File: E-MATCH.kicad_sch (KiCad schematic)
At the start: 22 parts, among them IC1 NCV81071BZR2G, IC2 NCV81071BZR2G, J1 691210910002, J2 691210910002, J3 691210910002, J4 691210910002, J5 DC Jack, Q1 AOSP36326C, Q2 AOSP36326C, Q3 AOSP36326C, Q4 AOSP36326C, U1 TMCS1108A2UQDR

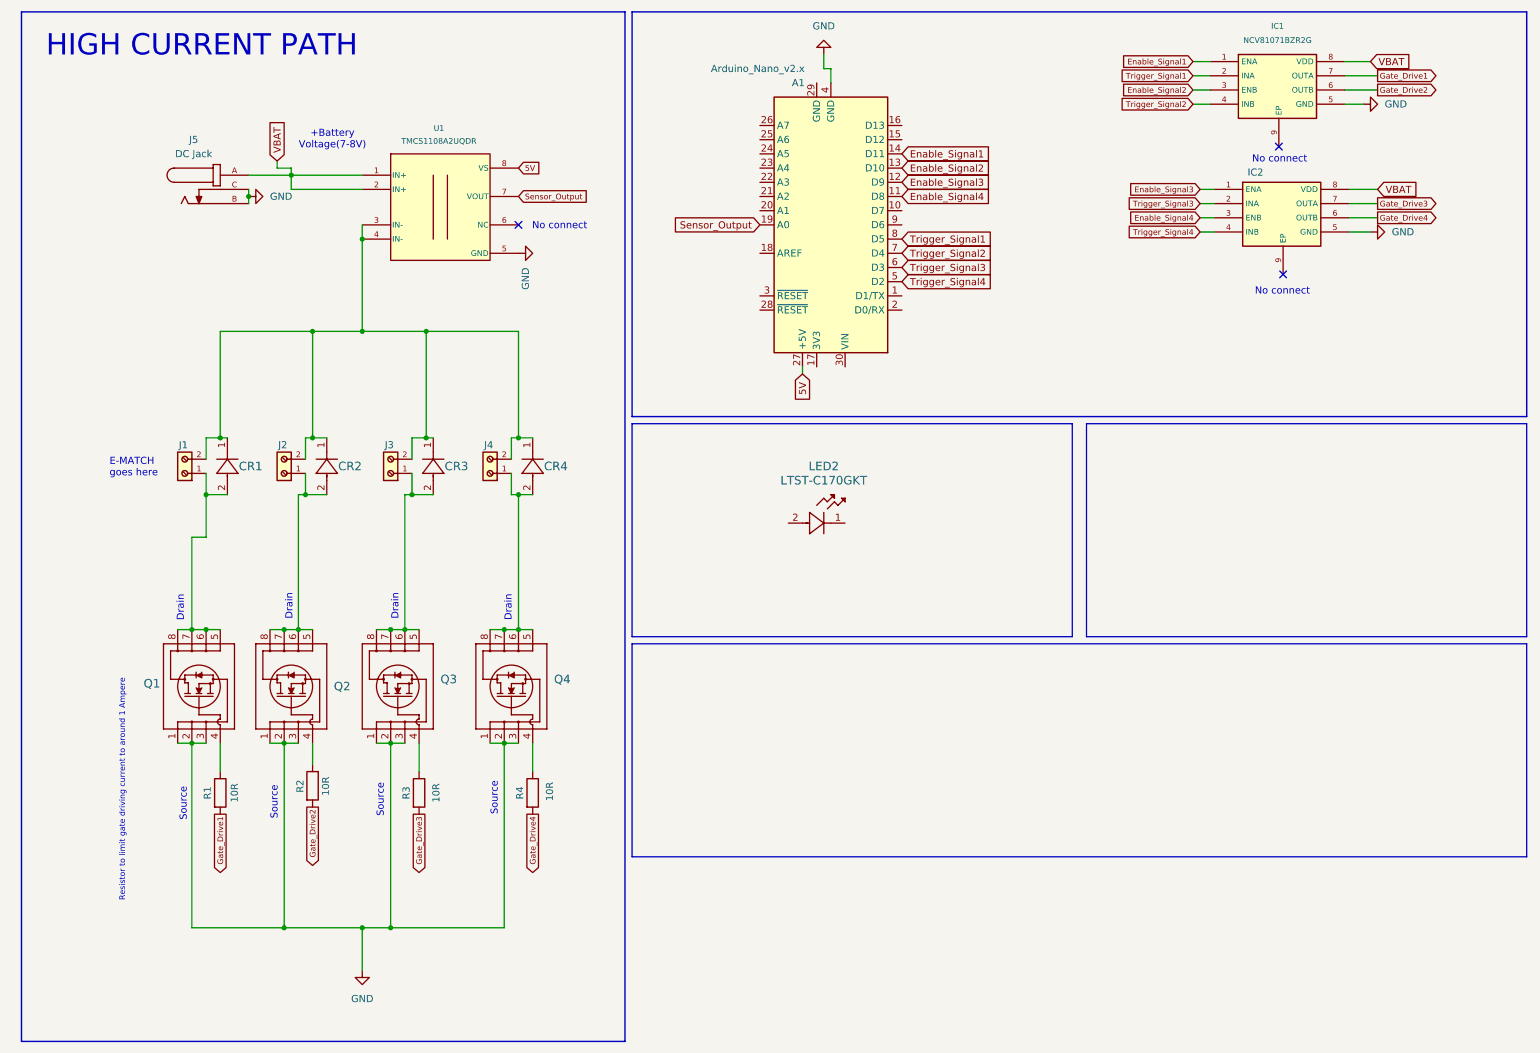
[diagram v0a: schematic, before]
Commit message: Schematic Cleanup
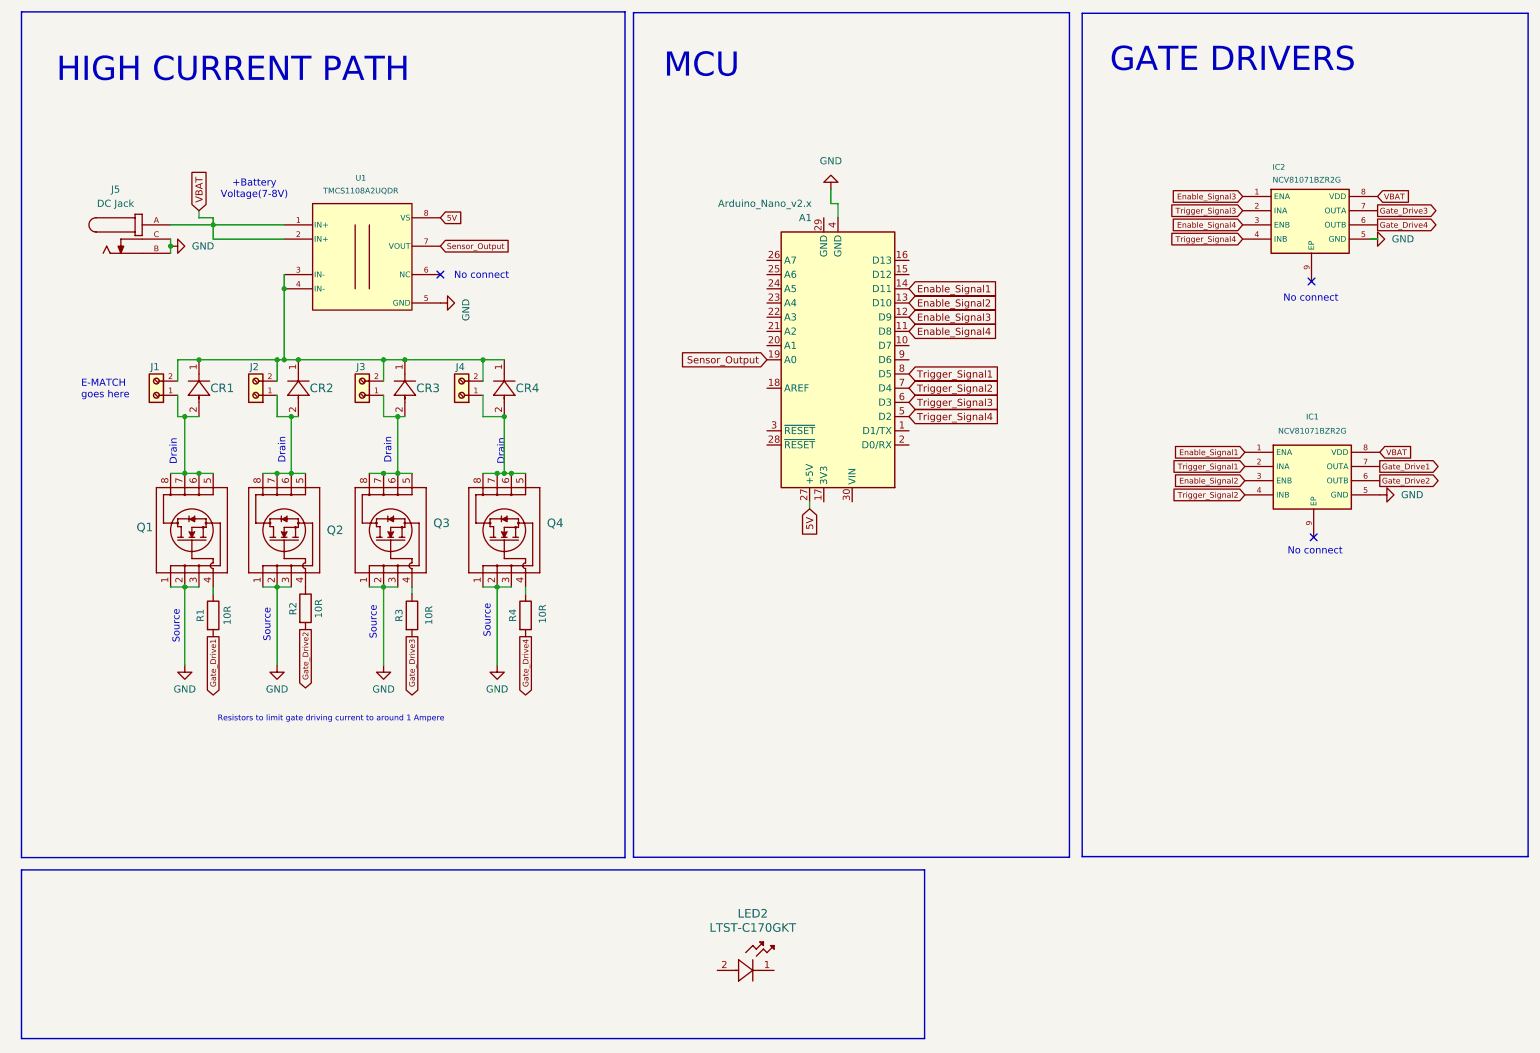
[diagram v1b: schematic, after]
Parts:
- IC2: footprint (none) -> SOP65P490X110-9N
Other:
- note added: "GATE DRIVERS"
- note added: "MCU"
- note added: "Resistors to limit gate driving current to around 1 Ampere"
- note removed: "Resistor to limit gate driving current to around 1 Ampere"
- moved on the sheet: A1, CR1, CR2, CR3, CR4, IC1, IC2, J1, J2, J3, J4, J5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
